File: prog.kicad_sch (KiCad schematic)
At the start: 43 parts, among them J3 USB_C_Receptacle, J4 probe_debug, SW1 BOOTSEL, SW2 RUN, U5 RP2040, U7 W25Q16JVSS, Y1 12 MHz

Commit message: jlc codes filled
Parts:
- R1, R7: jlc (none) -> C25804
- R10, R3, R4: jlc (none) -> C23186
- R2, R8: jlc (none) -> C21190
- R27, R28, R29, R30: jlc (none) -> C22775
- R5, R6: jlc (none) -> C25190
- U5: jlc (none) -> C2040
- U7: jlc (none) -> C131025
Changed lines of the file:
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@@
 			)
 		)
+		(property "jlc" "C25190"
+			(at 78.74 139.7 0)
+			(effects
+				(font
+					(size 1.27 1.27)
+				)
+				(hide yes)
+			)
+		)
 		(pin "1"
 		)
@@
 			)
 		)
+		(property "jlc" "C21190"
+			(at 40.64 38.1 0)
+			(effects
+				(font
+					(size 1.27 1.27)
+				)
+				(hide yes)
+			)
+		)
 		(pin "1"
 		)
@@
 			)
 		)
+		(property "jlc" "C23186"
+			(at 227.33 142.24 0)
+			(effects
+				(font
+					(size 1.27 1.27)
+				)
+				(hide yes)
+			)
+		)
 		(pin "1"
 		)
@@
 			)
 		)
+		(property "jlc" "C25190"
+			(at 78.74 142.24 0)
+			(effects
+				(font
+					(size 1.27 1.27)
+				)
+				(hide yes)
+			)
+		)
 		(pin "1"
 		)
@@
 			)
 		)
+		(property "jlc" "C21190"
+			(at 152.4 127 0)
+			(effects
+				(font
+					(size 1.27 1.27)
+				)
+				(hide yes)
+			)
+		)
 		(pin "1"
 		)
@@
 			)
 		)
+		(property "jlc" "C23186"
+			(at 58.42 132.08 0)
+			(effects
+				(font
+					(size 1.27 1.27)
+				)
+				(hide yes)
+			)
+		)
 		(pin "1"
 		)
@@
 			)
 		)
+		(property "jlc" "C25804"
+			(at 151.13 63.5 0)
+			(effects
+				(font
+					(size 1.27 1.27)
+				)
+				(hide yes)
+			)
+		)
 		(pin "1"
 		)
@@
 			)
 		)
+		(property "jlc" "C22775"
+			(at 219.71 74.93 0)
+			(effects
+				(font
+					(size 1.27 1.27)
+				)
+				(hide yes)
+			)
+		)
 		(pin "1"
 		)
@@
 			)
 		)
+		(property "jlc" "C22775"
+			(at 219.71 72.39 0)
+			(effects
+				(font
+					(size 1.27 1.27)
+				)
+				(hide yes)
+			)
+		)
 		(pin "1"
 		)
@@
 			)
 		)
+		(property "jlc" "C25804"
+			(at 50.8 38.1 0)
+			(effects
+				(font
+					(size 1.27 1.27)
+				)
+				(hide yes)
+			)
+		)
 		(pin "1"
 		)
@@
 			)
 		)
+		(property "jlc" "C131025"
+			(at 64.77 58.42 0)
+			(effects
+				(font
+					(size 1.27 1.27)
+				)
+				(hide yes)
+			)
+		)
 		(pin "1"
 		)
@@
 			)
 		)
+		(property "jlc" "C23186"
+			(at 58.42 129.54 0)
+			(effects
+				(font
+					(size 1.27 1.27)
+				)
+				(hide yes)
+			)
+		)
 		(pin "1"
 		)
@@
 			)
 		)
+		(property "jlc" "C22775"
+			(at 266.7 71.12 0)
+			(effects
+				(font
+					(size 1.27 1.27)
+				)
+				(hide yes)
+			)
+		)
 		(pin "1"
 		)
@@
 			)
 		)
+		(property "jlc" "C2040"
+			(at 187.96 105.41 0)
+			(effects
+				(font
+					(size 1.27 1.27)
+				)
+				(hide yes)
+			)
+		)
 		(pin "16"
 		)
@@
 			(at 266.7 86.36 0)
 			(effects
+				(font
+					(size 1.27 1.27)
+				)
+				(hide yes)
+			)
+		)
+		(property "jlc" "C22775"
+			(at 266.7 86.36 0)
+			(effects

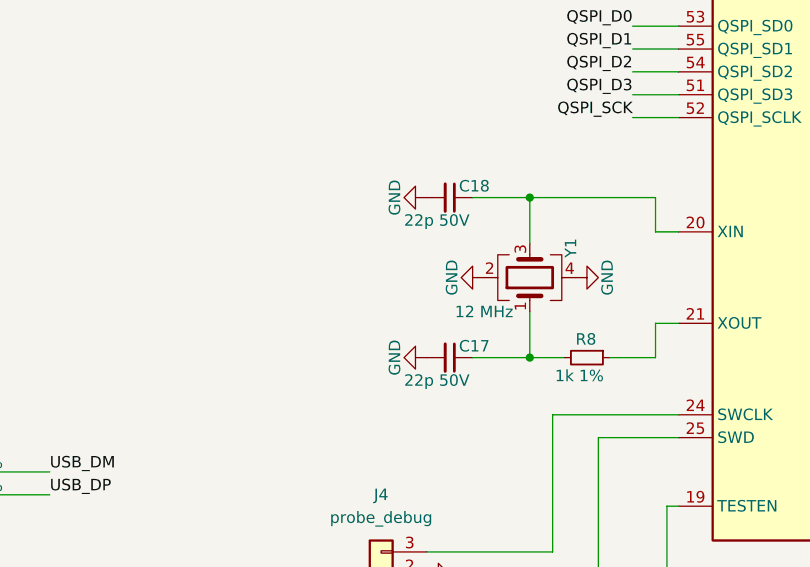
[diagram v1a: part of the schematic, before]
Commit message: routing in progress
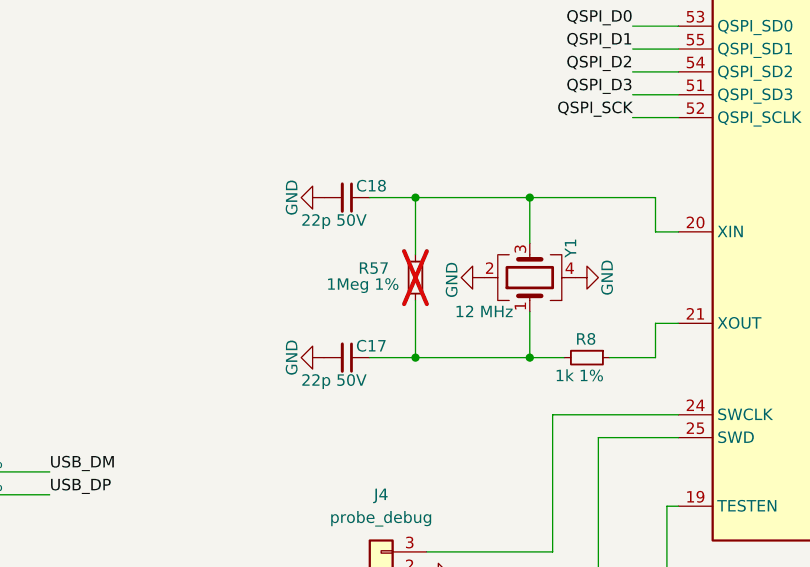
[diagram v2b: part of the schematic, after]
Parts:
- added R57: 1Meg 1%, Resistor_SMD:R_0603_1608Metric_Pad0.98x0.95mm_HandSolder, symbol Device:R_Small
- R7: now left out of the parts list
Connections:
- net at C17.1, R8.2, Y1.1: now also R57.2
- net at C18.1, U5.20 (XIN), Y1.3: now also R57.1
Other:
- moved on the sheet: C17, C18
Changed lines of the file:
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@@
 	)
 	(junction
+		(at 133.35 109.22)
+		(diameter 0)
+		(color 0 0 0 0)
+	)
+	(junction
 		(at 151.13 67.31)
 		(diameter 0)
@@
 	)
 	(junction
+		(at 133.35 127)
+		(diameter 0)
+		(color 0 0 0 0)
+	)
+	(junction
 		(at 80.01 73.66)
 		(diameter 0)
@@
 	(wire
 		(pts
-			(xy 139.7 109.22) (xy 146.05 109.22)
+			(xy 128.27 109.22) (xy 133.35 109.22)
 		)
 		(stroke
@@
 	(wire
 		(pts
+			(xy 133.35 109.22) (xy 133.35 115.57)
+		)
+		(stroke
+			(width 0)
+			(type default)
+		)
+	)
+	(wire
+		(pts
 			(xy 60.96 129.54) (xy 68.58 129.54)
 		)
@@
 	(wire
 		(pts
+			(xy 133.35 120.65) (xy 133.35 127)
+		)
+		(stroke
+			(width 0)
+			(type default)
+		)
+	)
+	(wire
+		(pts
 			(xy 52.07 132.08) (xy 55.88 132.08)
 		)
@@
 	(wire
 		(pts
+			(xy 133.35 109.22) (xy 146.05 109.22)
+		)
+		(stroke
+			(width 0)
+			(type default)
+		)
+	)
+	(wire
+		(pts
 			(xy 154.94 127) (xy 160.02 127)
 		)
@@
 	(wire
 		(pts
+			(xy 133.35 127) (xy 128.27 127)
+		)
+		(stroke
+			(width 0)
+			(type default)
+		)
+	)
+	(wire
+		(pts
 			(xy 256.54 71.12) (xy 261.62 71.12)
 		)
@@
 	(wire
 		(pts
-			(xy 146.05 127) (xy 139.7 127)
+			(xy 146.05 127) (xy 133.35 127)
 		)
 		(stroke
@@
 	(symbol
 		(lib_id "power:GND")
-		(at 134.62 109.22 270)
+		(at 123.19 109.22 270)
 		(unit 1)
 		(exclude_from_sim no)
@@
 		(dnp no)
 		(property "Reference" "#PWR061"
-			(at 128.27 109.22 0)
+			(at 116.84 109.22 0)
 			(effects
 				(font
@@
 		)
 		(property "Value" "GND"
-			(at 131.064 109.22 0)
+			(at 119.634 109.22 0)
 			(effects
 				(font
@@
 		)
 		(property "Footprint" ""
-			(at 134.62 109.22 0)
+			(at 123.19 109.22 0)
 			(effects
 				(font
@@
 		)
 		(property "Datasheet" ""
-			(at 134.62 109.22 0)
+			(at 123.19 109.22 0)
 			(effects
 				(font
@@
 		)
 		(property "Description" "Power symbol creates a global label with name \"GND\" , ground"
-			(at 134.62 109.22 0)
+			(at 123.19 109.22 0)
 			(effects
 				(font
@@
 		)
 		(property "Value" "GND"
-			(at 137.414 118.11 0)
+			(at 137.414 118.364 0)
 			(effects
 				(font
@@
 		(unit 1)
 		(exclude_from_sim no)
-		(in_bom yes)
+		(in_bom no)
 		(on_board yes)
 		(dnp yes)
@@
 	(symbol
 		(lib_id "Device:C_Small")
-		(at 137.16 127 270)
+		(at 125.73 127 270)
 		(unit 1)
 		(exclude_from_sim no)
@@
 		(dnp no)
 		(property "Reference" "C17"
-			(at 138.176 125.73 90)
+			(at 126.746 125.73 90)
 			(effects
 				(font
@@
 		)
 		(property "Value" "22p 50V"
-			(at 132.08 129.54 90)
+			(at 120.65 129.54 90)
 			(effects
 				(font
@@
 		)
 		(property "Footprint" "Capacitor_SMD:C_0603_1608Metric_Pad1.08x0.95mm_HandSolder"
-			(at 137.16 127 0)
+			(at 125.73 127 0)
 			(effects
 				(font
@@
 		)
 		(property "Datasheet" "~"
-			(at 137.16 127 0)
+			(at 125.73 127 0)
 			(effects
 				(font
@@
 		)
 		(property "Description" ""
-			(at 137.16 127 0)
+			(at 125.73 127 0)
 			(effects
 				(font
@@
 		)
 		(property "jlc" "C1653"
-			(at 137.16 127 90)
+			(at 125.73 127 90)
 			(effects
 				(font
@@
 	)
 	(symbol
+		(lib_id "Device:R_Small")
+		(at 133.35 118.11 0)
+		(unit 1)
+		(exclude_from_sim no)
+		(in_bom no)
+		(on_board yes)
+		(dnp yes)
+		(property "Reference" "R57"
+			(at 127 117.094 0)
+			(effects
+				(font
+					(size 1.27 1.27)
+				)
+				(justify left)
+			)
+		)
+		(property "Value" "1Meg 1%"
+			(at 123.444 118.872 0)
+			(effects
+				(font
+					(size 1.27 1.27)
+				)
+				(justify left)
+			)
+		)
+		(property "Footprint" "Resistor_SMD:R_0603_1608Metric_Pad0.98x0.95mm_HandSolder"
+			(at 133.35 118.11 0)
+			(effects
+				(font
+					(size 1.27 1.27)
+				)
+				(hide yes)
+			)
+		)
+		(property "Datasheet" "~"
+			(at 133.35 118.11 0)
+			(effects
+				(font
+					(size 1.27 1.27)
+				)
+				(hide yes)
+			)
+		)
+		(property "Description" ""
+			(at 133.35 118.11 0)
+			(effects
+				(font
+					(size 1.27 1.27)
+				)
+				(hide yes)
+			)
+		)
+		(property "jlc" ""
+			(at 133.35 118.11 0)
+			(effects
+				(font
+					(size 1.27 1.27)
+				)
+				(hide yes)
+			)
+		)
+		(pin "1"
+		)
+		(pin "2"
+		)
+		(instances
+			(project "beam_kit_1"
+				(path "/3a707576-1044-44db-8cf8-deb84fe605c8/35bb5101-2bc6-4b84-84b4-e3f71c5fc9a9"
+					(reference "R57")
+					(unit 1)
+				)
+			)
+		)
+	)
+	(symbol
 		(lib_id "Connector_Generic:Conn_01x03")
 		(at 129.54 151.13 180)
@@
 	(symbol
 		(lib_id "Device:C_Small")
-		(at 137.16 109.22 270)
+		(at 125.73 109.22 270)
 		(unit 1)
 		(exclude_from_sim no)
@@
 		(dnp no)
 		(property "Reference" "C18"
-			(at 138.176 107.95 90)
+			(at 126.746 107.95 90)
 			(effects
 				(font
@@
 		)
 		(property "Value" "22p 50V"
-			(at 132.08 111.76 90)
+			(at 120.65 111.76 90)
 			(effects
 				(font
@@
 		)
 		(property "Footprint" "Capacitor_SMD:C_0603_1608Metric_Pad1.08x0.95mm_HandSolder"
-			(at 137.16 109.22 0)
+			(at 125.73 109.22 0)
 			(effects
 				(font
@@
 		)
 		(property "Datasheet" "~"
-			(at 137.16 109.22 0)
+			(at 125.73 109.22 0)
 			(effects
 				(font
@@
 		)
 		(property "Description" ""
-			(at 137.16 109.22 0)
+			(at 125.73 109.22 0)
 			(effects
 				(font
@@
 		)
 		(property "jlc" "C1653"
-			(at 137.16 109.22 90)
+			(at 125.73 109.22 90)
 			(effects
 				(font
@@
 	(symbol
 		(lib_id "power:GND")
-		(at 134.62 127 270)
+		(at 123.19 127 270)
 		(unit 1)
 		(exclude_from_sim no)
@@
 		(dnp no)
 		(property "Reference" "#PWR062"
-			(at 128.27 127 0)
+			(at 116.84 127 0)
 			(effects
 				(font
@@
 		)
 		(property "Value" "GND"
-			(at 131.064 127 0)
+			(at 119.634 127 0)
 			(effects
 				(font
@@
 		)
 		(property "Footprint" ""
-			(at 134.62 127 0)
+			(at 123.19 127 0)
 			(effects
 				(font
@@
 		)
 		(property "Datasheet" ""
-			(at 134.62 127 0)
+			(at 123.19 127 0)
 			(effects
 				(font
@@
 		)
 		(property "Description" "Power symbol creates a global label with name \"GND\" , ground"
-			(at 134.62 127 0)
+			(at 123.19 127 0)
 			(effects
 				(font
